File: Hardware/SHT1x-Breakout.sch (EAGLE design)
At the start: 9 parts, among them U1 SHT1XSMD

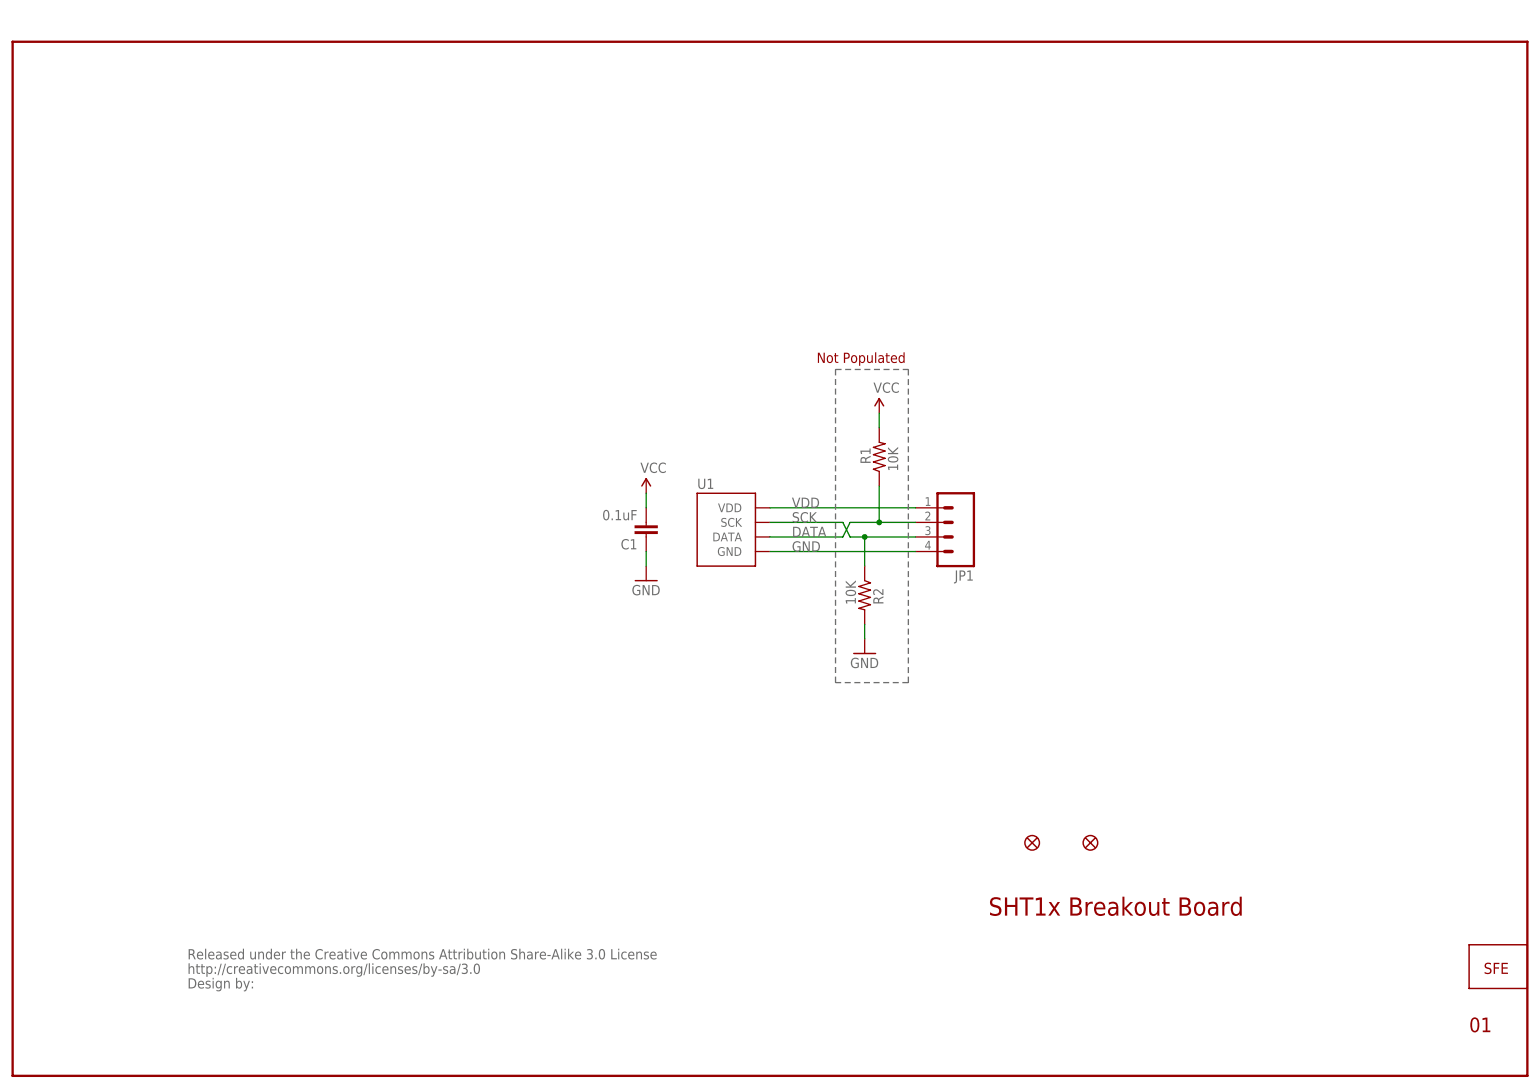
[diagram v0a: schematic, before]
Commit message: Initial Revision Commit
Testing to make sure changes only happen to V_1.4 branch. Initial
layout of new revision.
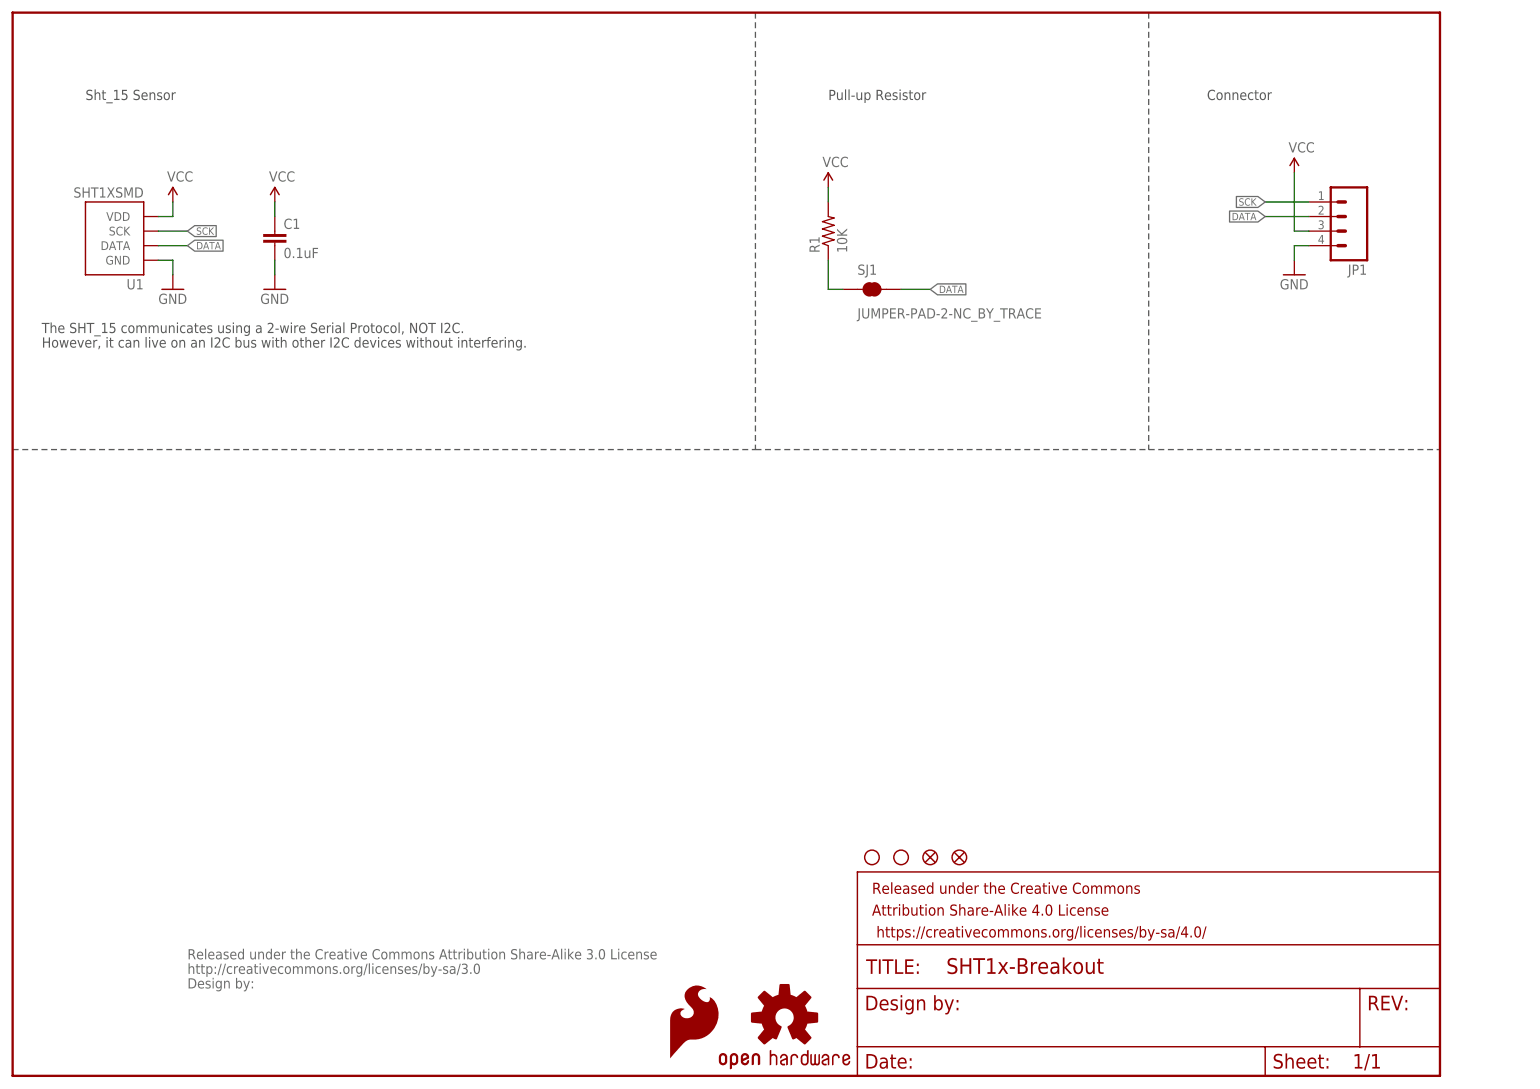
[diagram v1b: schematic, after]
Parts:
- removed R2: 10K, SparkFun:RESISTOR0603-RES
- removed U$1: LOGO-SFENEW, SparkFun:LOGO-SFENEW
- removed U$2, U$3: FIDUCIAL1X2, SparkFun:FIDUCIAL1X2
- added FID1, FID2: FIDUCIAL1X2, SparkFun-Aesthetics:FIDUCIAL1X2
- added FRAME1: (no value), SparkFun-Aesthetics:FRAME-LETTER
- added LOGO1: OSHW-LOGOS, SparkFun-Aesthetics:OSHW-LOGOS
- added LOGO4: SFE_LOGO_FLAME.1_INCH, SparkFun-Aesthetics:SFE_LOGO_FLAME.1_INCH
- added SJ1: JUMPER-PAD-2-NC_BY_TRACE, SparkFun-Passives:JUMPER-PAD-2-NC_BY_TRACE
- added STANDOFF1, STANDOFF2: STAND-OFF, SparkFun-Electromechanical:STAND-OFF
- C1: device SparkFun:CAP0603-CAP -> SparkFun-Capacitors:0.1UF-25V(+80/-20%)(0603)
- R1: device SparkFun:RESISTOR0603-RES -> SparkFun-Resistors:10KOHM-1/10W-1%(0603)0603
- U1: device SparkFun:SHT1XSMD -> SparkFun-Sensors:SHT1XSMD
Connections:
- removed net VDD: C1.2, JP1.1, R1.2, U1.VDD
- new net N$1: R1.1, SJ1.1
- new net VCC: C1.1, JP1.3, R1.2, U1.VDD
- net DATA: now also SJ1.2; no longer R1.1
- net GND: now also C1.2; no longer C1.1, R2.2
- net SCK: now also JP1.1; no longer JP1.3, R2.1
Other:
- note added: "Connector"
- note added: "However, it can live on an I2C bus with other I2C devices without interfering."
- note added: "Pull-up Resistor"
- note added: "Sht_15 Sensor"
- note added: "The SHT_15 communicates using a 2-wire Serial Protocol, NOT I2C."
- note removed: "01"
- note removed: "Not Populated"
- note removed: "SHT1x Breakout Board"
- moved on the sheet: C1, JP1, R1, U1
